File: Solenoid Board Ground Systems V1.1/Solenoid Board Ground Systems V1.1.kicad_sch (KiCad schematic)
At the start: 27 parts, among them J1 OUT CHAN A, J2 POWER IN, J3 OUT CHAN B

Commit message: Changed all the things to 5mm pitch
yuck big board be like
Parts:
- J1, J3: footprint TerminalBlock_Phoenix:TerminalBlock_Phoenix_MPT-0,5-8-2.54_1x08_P2.54mm_Horizontal -> TerminalBlock_Phoenix:TerminalBlock_Phoenix_PT-1,5-8-5.0-H_1x08_P5.00mm_Horizontal
- J2: footprint TerminalBlock_Phoenix:TerminalBlock_Phoenix_MPT-0,5-9-2.54_1x09_P2.54mm_Horizontal -> TerminalBlock_Phoenix:TerminalBlock_Phoenix_PT-1,5-9-5.0-H_1x09_P5.00mm_Horizontal

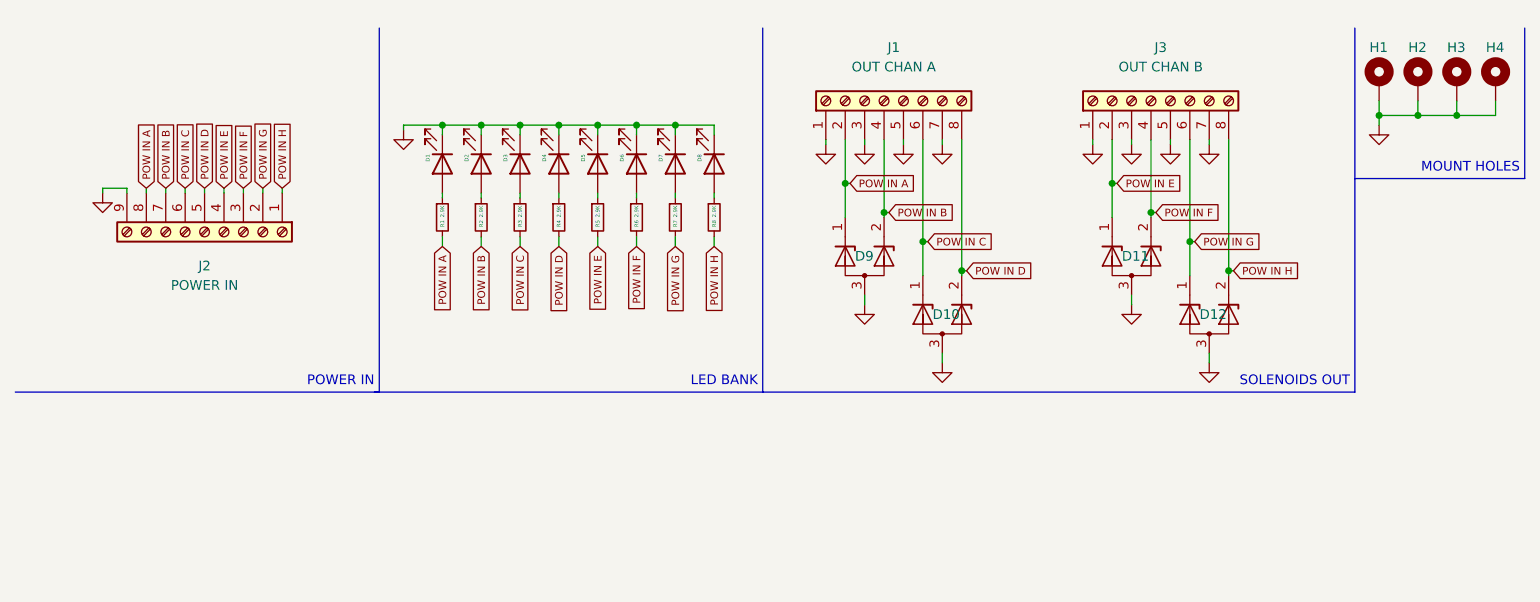
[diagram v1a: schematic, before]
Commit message: Revions and new board
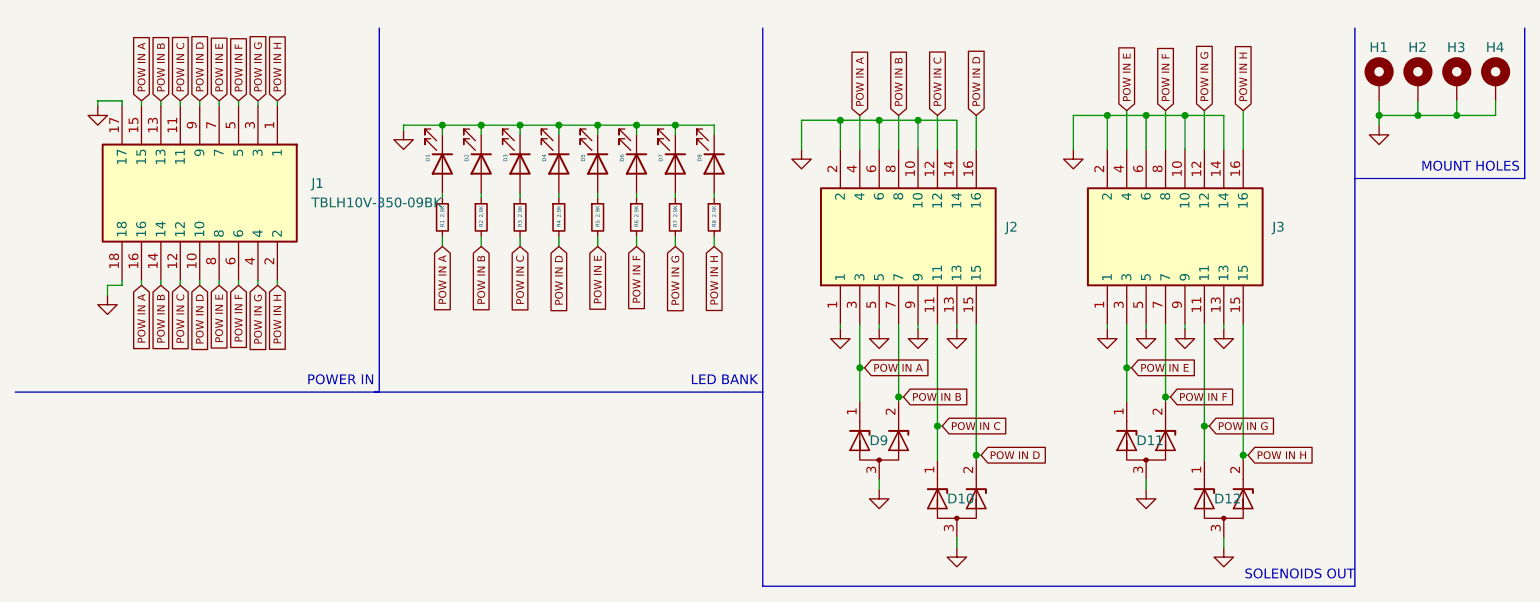
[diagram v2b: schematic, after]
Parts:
- removed J1: OUT CHAN A, TerminalBlock_Phoenix:TerminalBlock_Phoenix_PT-1,5-8-5.0-H_1x08_P5.00mm_Horizontal, symbol Connector:Screw_Terminal_01x08
- removed J2: POWER IN, TerminalBlock_Phoenix:TerminalBlock_Phoenix_PT-1,5-9-5.0-H_1x09_P5.00mm_Horizontal, symbol Connector:Screw_Terminal_01x09
- removed J3: OUT CHAN B, TerminalBlock_Phoenix:TerminalBlock_Phoenix_PT-1,5-8-5.0-H_1x08_P5.00mm_Horizontal, symbol Connector:Screw_Terminal_01x08
- added J1: TBLH10V-350-09BK, RHDR18W80P550X350_2X9_3220X850X1420P, symbol TBLH10V-350-09BK:TBLH10V-350-09BK
- added J2, J3: TBLH10V-350-08BK, RHDR16W80P550X350_2X8_2870X850X1420P, symbol TBLH10V-350-08BK:TBLH10V-350-08BK
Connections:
- net GND: now also J1.17, J1.18, J2.1, J2.10, J2.13, J2.14, J2.2, J2.5, J2.6, J2.9, J3.1, J3.10, J3.13, J3.14, J3.2, J3.5, J3.6, J3.9
- net POW IN A: now also J1.15, J1.16, J2.3, J2.4
- net POW IN B: now also J1.13, J1.14, J2.7, J2.8
- net POW IN C: now also J1.11, J1.12, J2.11, J2.12
- net POW IN D: now also J1.10, J1.9, J2.15, J2.16
- net POW IN E: now also J1.7, J1.8, J3.3, J3.4
- net POW IN F: now also J1.5, J1.6, J3.7, J3.8
- net POW IN G: now also J1.3, J1.4, J3.11, J3.12
- net POW IN H: now also J1.1, J1.2, J3.15, J3.16
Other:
- moved on the sheet: D10, D11, D12, D9
